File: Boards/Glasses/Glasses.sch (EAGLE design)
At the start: 256 parts, among them U1 APA1022020, U10 APA1022020, U100 APA1022020, U101 APA1022020, U102 APA1022020, U103 APA1022020, U104 APA1022020, U105 APA1022020, U106 APA1022020, U107 APA1022020, U108 APA1022020, U109 APA1022020, U11 APA1022020, U110 APA1022020, U111 APA1022020, U112 APA1022020, U113 APA1022020, U114 APA1022020, U115 APA1022020, U116 APA1022020, U117 APA1022020, U118 APA1022020, U119 APA1022020, U12 APA1022020, U120 APA1022020, U121 APA1022020, U122 APA1022020, U123 APA1022020, U124 APA1022020, U125 APA1022020, U126 APA1022020, U127 APA1022020, U128 APA1022020, U129 APA1022020, U13 APA1022020, U130 APA1022020, U131 APA1022020, U132 APA1022020, U133 APA1022020, U134 APA1022020, U135 APA1022020, U136 APA1022020, U137 APA1022020, U138 APA1022020, U139 APA1022020, U14 APA1022020, U140 APA1022020, U141 APA1022020, U142 APA1022020, U143 APA1022020, U144 APA1022020, U145 APA1022020, U146 APA1022020, U147 APA1022020, U148 APA1022020, U149 APA1022020, U15 APA1022020, U150 APA1022020, U151 APA1022020, U152 APA1022020, U153 APA1022020, U154 APA1022020, U155 APA1022020, U156 APA1022020, U157 APA1022020, U158 APA1022020, U159 APA1022020, U16 APA1022020, U160 APA1022020, U161 APA1022020, U162 APA1022020, U163 APA1022020, U164 APA1022020, U165 APA1022020, U166 APA1022020, U167 APA1022020, U168 APA1022020, U169 APA1022020, U17 APA1022020, U170 APA1022020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

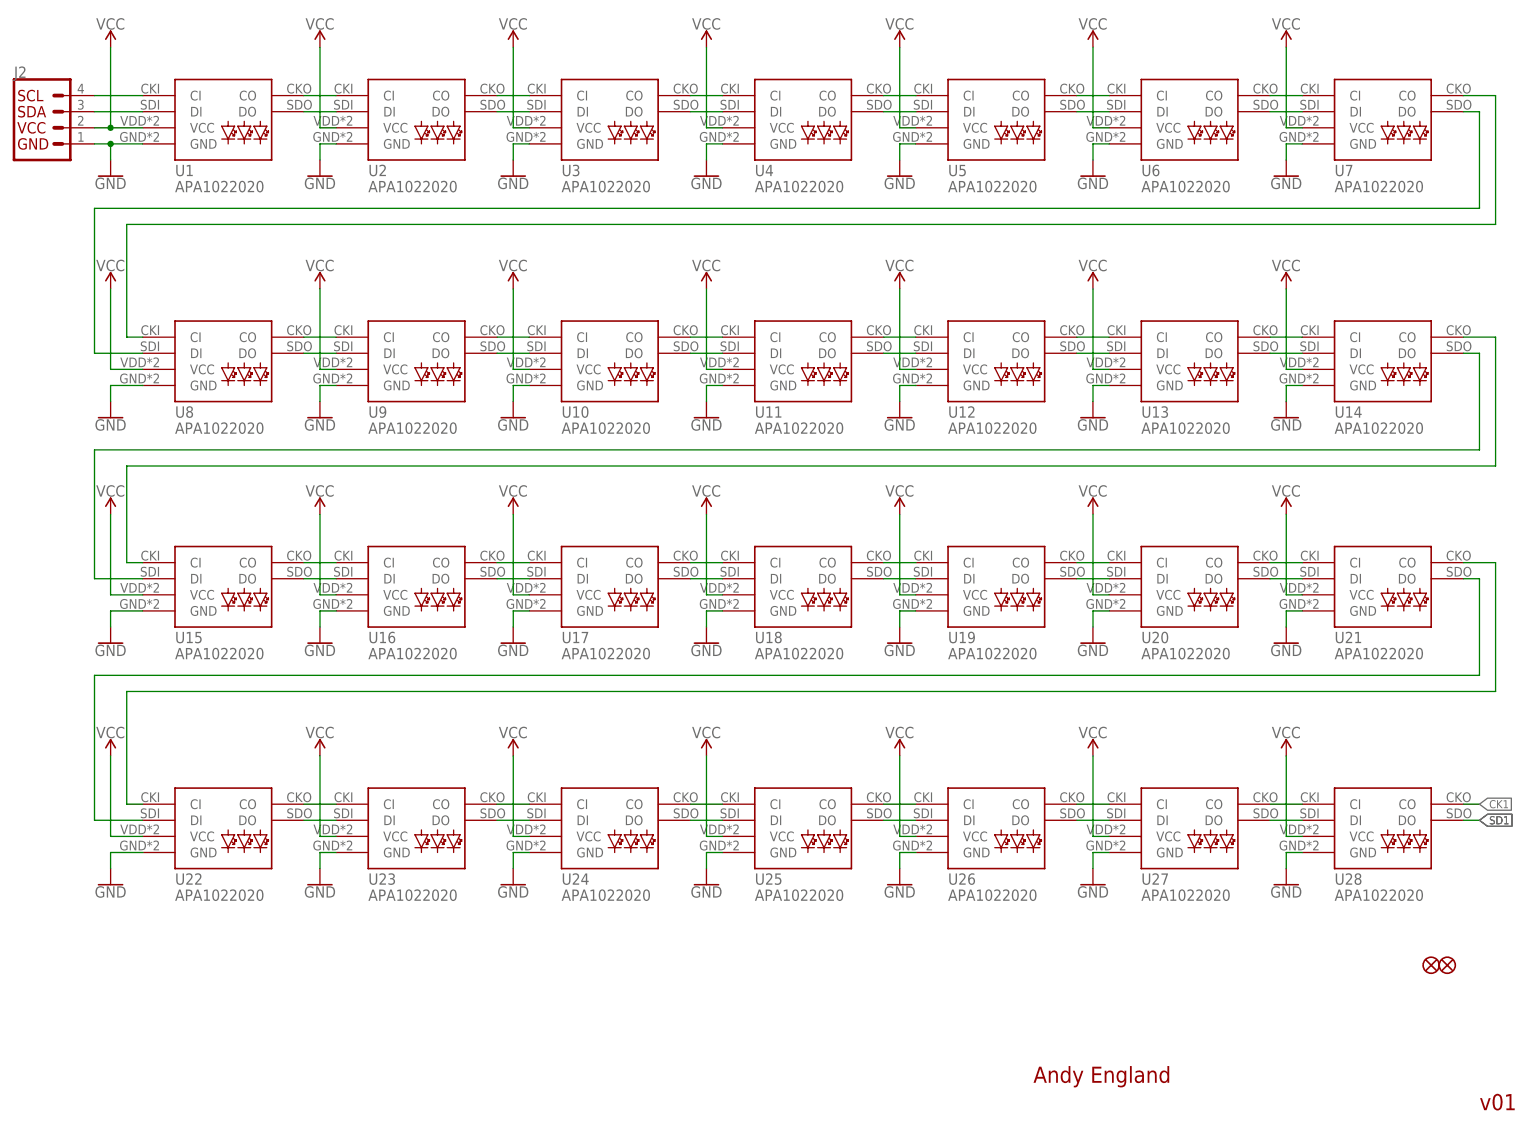
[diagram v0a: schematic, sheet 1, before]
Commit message: adding gcode
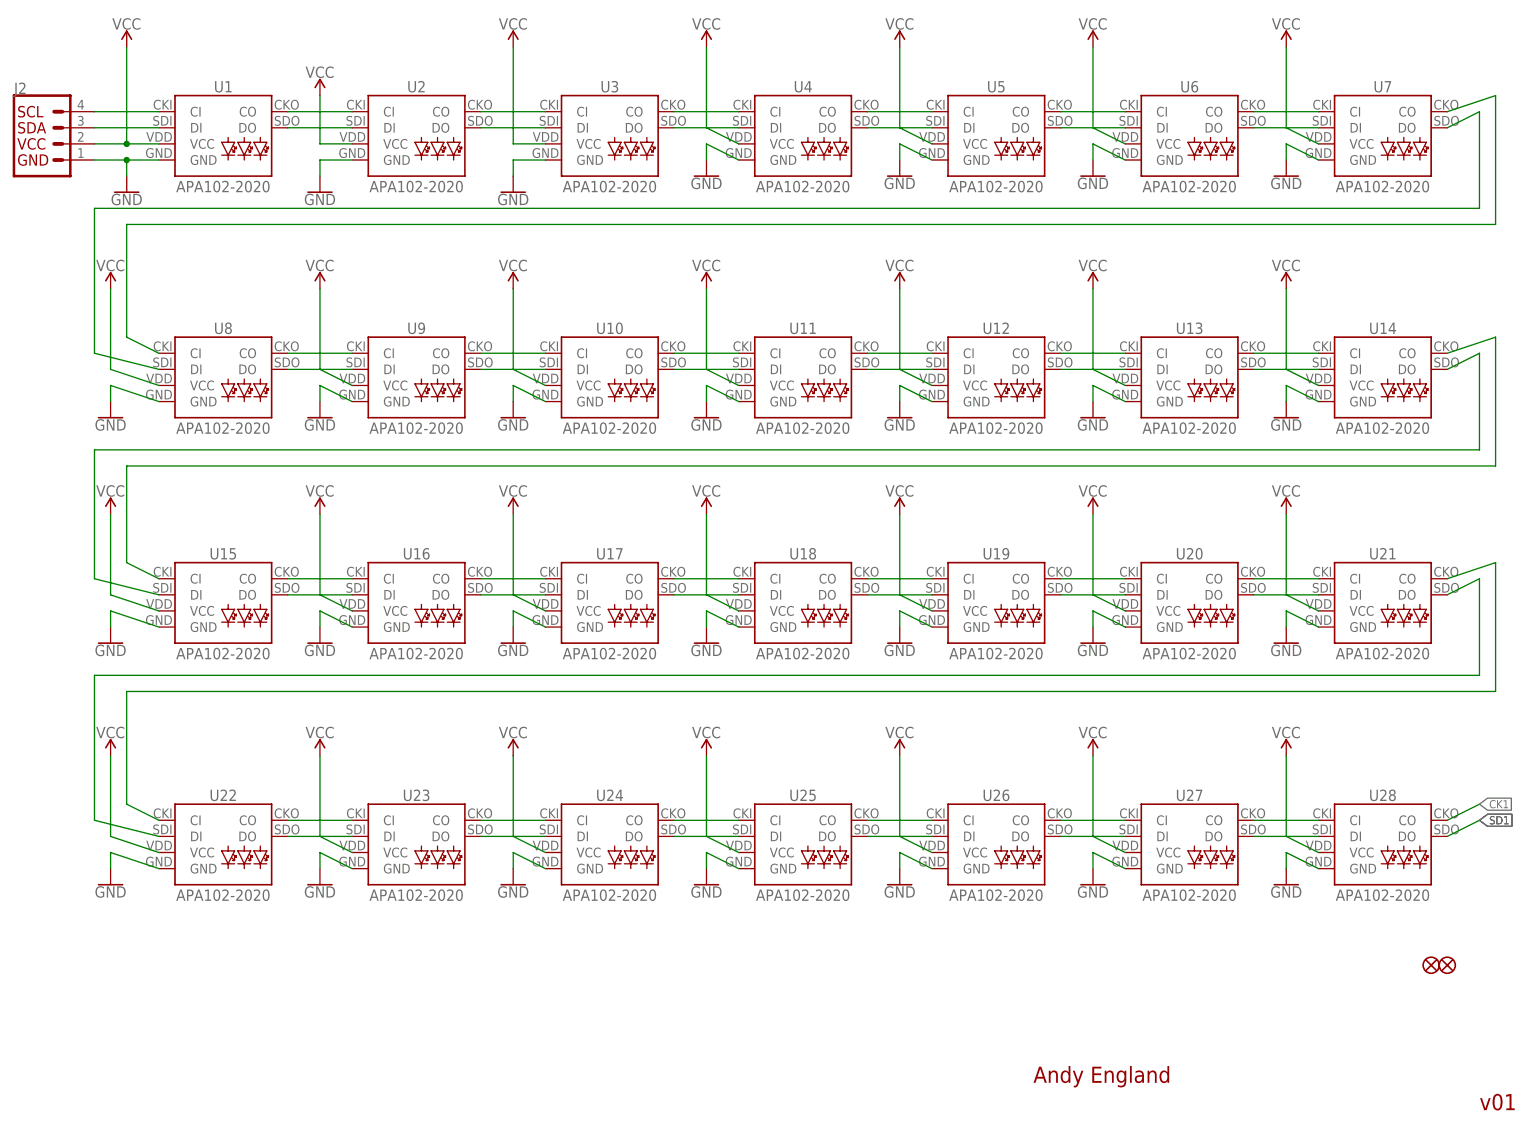
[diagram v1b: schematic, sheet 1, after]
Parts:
- U1, U10, U100, U101, U102, U103, U104, U105, U106, U107, U108, U109, U11, U110, U111, U112, U113, U114, U115, U116, U117, U118, U119, U12, U120, U121, U122, U123, U124, U125, U126, U127, U128, U129, U13, U130, U131, U132, U133, U134, U135, U136, U137, U138, U139, U14, U140, U141, U142, U143, U144, U145, U146, U147, U148, U149, U15, U150, U151, U152, U153, U154, U155, U156, U157, U158, U159, U16, U160, U161, U162, U163, U164, U165, U166, U167, U168, U169, U17, U170, U171, U172, U173, U174, U175, U176, U177, U178, U179, U18, U180, U181, U182, U183, U184, U185, U186, U187, U188, U189, U19, U190, U191, U192, U193, U194, U195, U196, U197, U198, U199, U2, U20, U200, U201, U202, U203, U204, U205, U206, U207, U208, U209, U21, U210, U211, U212, U213, U214, U215, U216, U217, U218, U219, U22, U220, U221, U222, U223, U224, U225, U226, U227, U228, U229, U23, U230, U231, U232, U233, U234, U235, U236, U237, U238, U239, U24, U240, U241, U242, U243, U244, U245, U246, U247, U248, U249, U25, U250, U251, U252, U26, U27, U28, U29, U3, U30, U31, U32, U33, U34, U35, U36, U37, U38, U39, U4, U40, U41, U42, U43, U44, U45, U46, U47, U48, U49, U5, U50, U51, U52, U53, U54, U55, U56, U57, U58, U59, U6, U60, U61, U62, U63, U64, U65, U66, U67, U68, U69, U7, U70, U71, U72, U73, U74, U75, U76, U77, U78, U79, U8, U80, U81, U82, U83, U84, U85, U86, U87, U88, U89, U9, U90, U91, U92, U93, U94, U95, U96, U97, U98, U99: value APA1022020 -> APA102-2020; device 1_BES_Optoelectronics:APA1022020 -> SparkFun-LED:APA102-2020
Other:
- moved on the sheet: J2, U1, U10, U100, U101, U102, U103, U104, U105, U106, U107, U108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
